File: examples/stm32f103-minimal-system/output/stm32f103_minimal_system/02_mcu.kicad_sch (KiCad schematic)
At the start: 7 parts, among them SW1 SW-TH_6x6, U1 STM32F103C8T6, Y1 8MHz

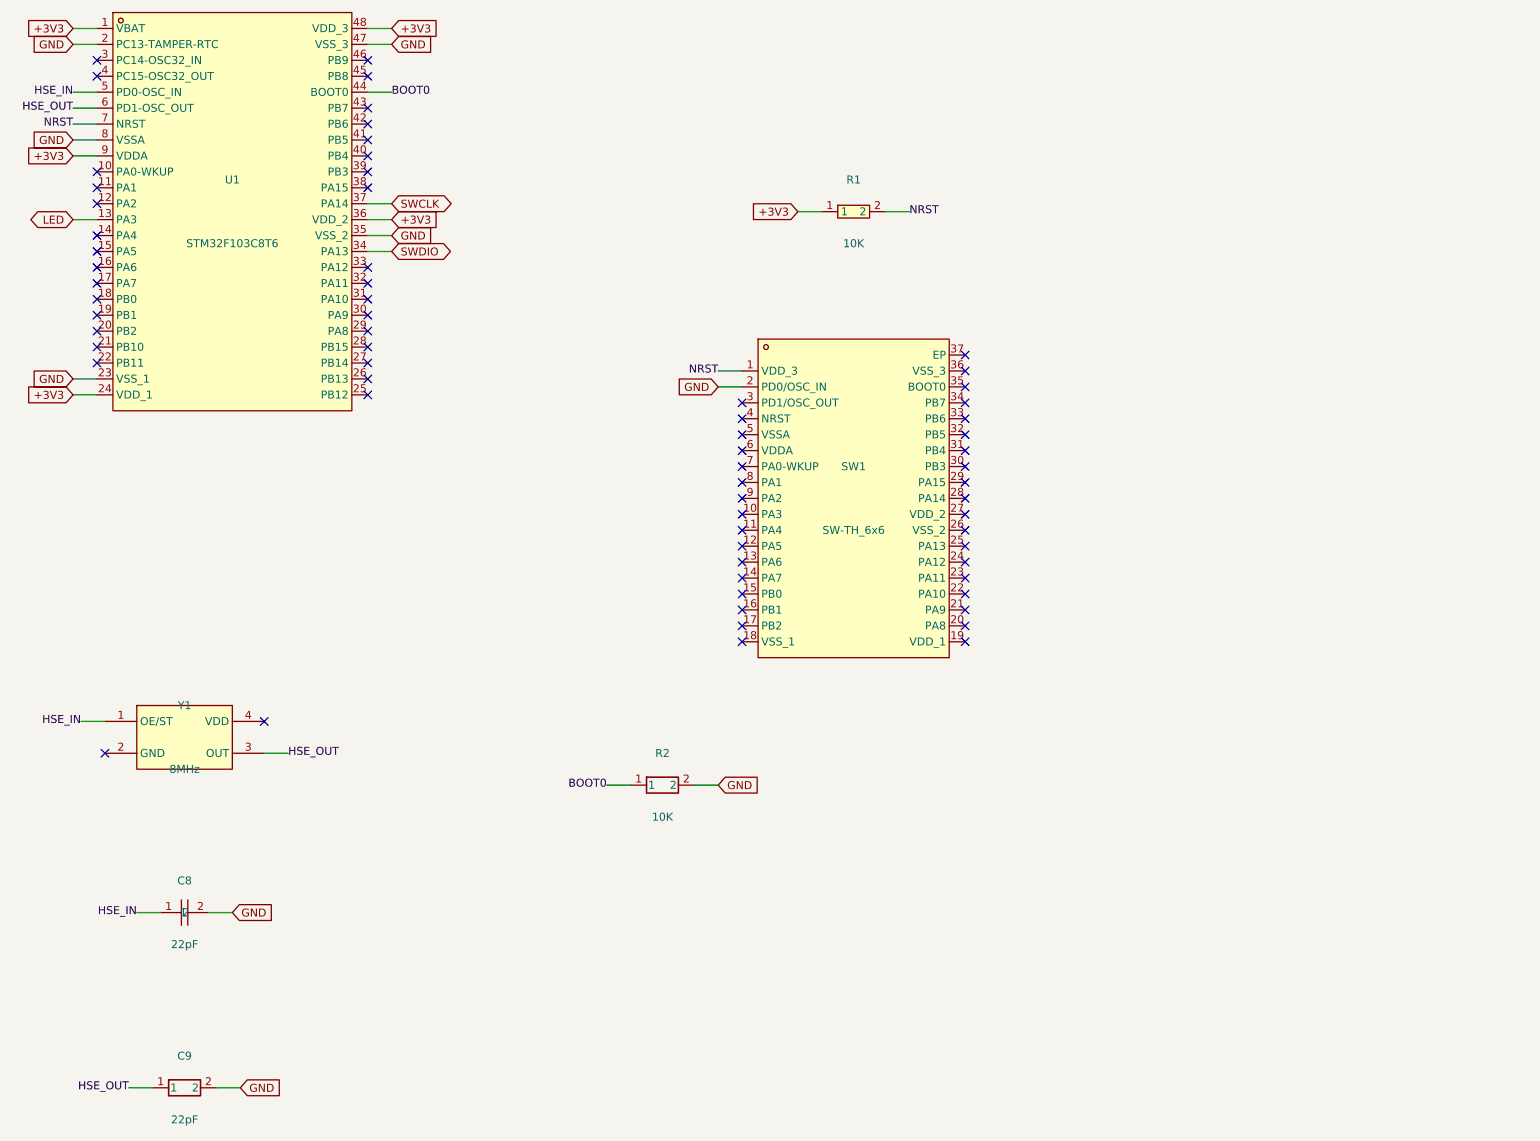
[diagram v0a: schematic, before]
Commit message: docs: refresh verified examples / 文档：刷新已验证示例
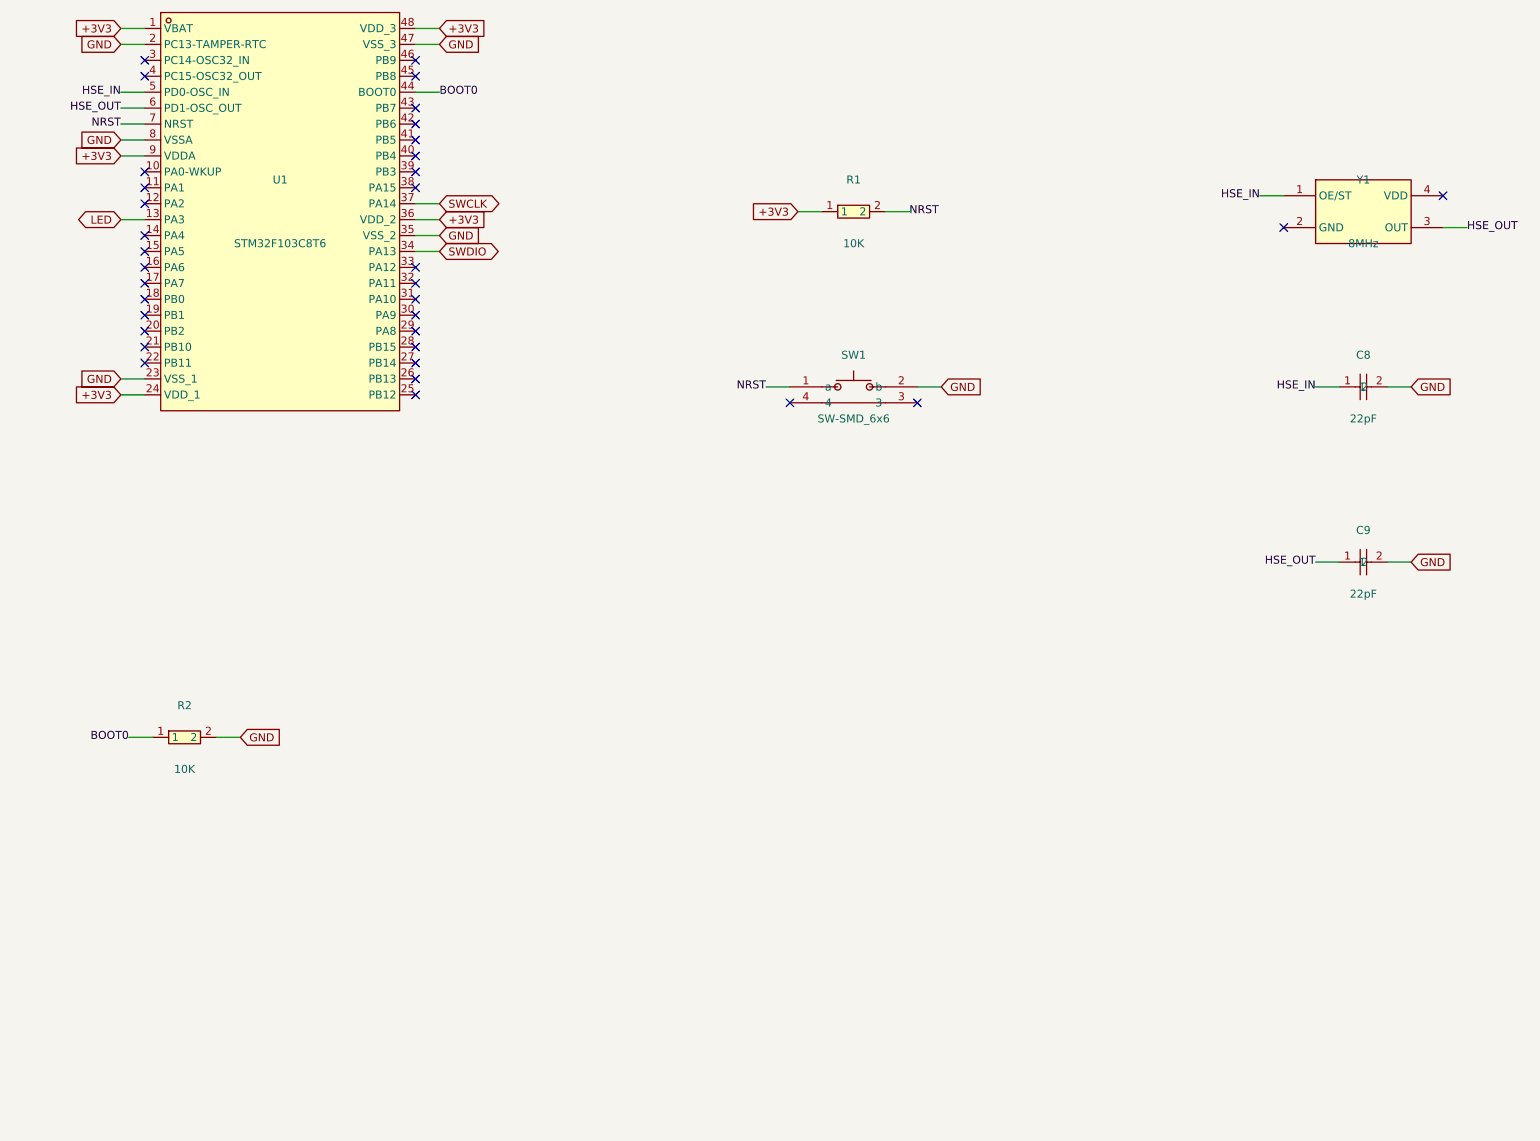
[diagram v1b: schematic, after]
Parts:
- removed C9: 22pF, symbol JLC-MCP:C1653
- removed R2: 10K, symbol JLC-MCP:C15401
- removed SW1: SW-TH_6x6, symbol JLC-MCP:STM32F103TBU6
- added C9: 22pF, JLC-MCP:C0603, symbol JLC-MCP:CL10C220JB8NNNC
- added R2: 10K, JLC-MCP:R0603, symbol JLC-MCP:0603WAJ0103T5E
- added SW1: SW-SMD_6x6, JLC-MCP:SW-SMD_K5-1617SA-02, symbol JLC-MCP:K5-1617SA-02
- C8: footprint (none) -> JLC-MCP:C0603
- R1: footprint (none) -> JLC-MCP:R0603
- U1: footprint (none) -> JLC-MCP:LQFP-48_L7.0-W7.0-P0.50-LS9.0-BL
- Y1: footprint (none) -> JLC-MCP:OSC-SMD_4P-L3.2-W2.5-BL
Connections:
- net BOOT0: now also R2.1
- net GND: now also C9.2, R2.2, SW1.2 (b)
- net HSE_OUT: now also C9.1
- net NRST: now also SW1.1 (a)
- no-connect marks 68 -> 35
